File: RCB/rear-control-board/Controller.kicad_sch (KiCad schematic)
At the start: 26 parts, among them J6 Conn_01x05, U1 STM32F413CGUx, U2 LD1117S33TR_SOT223, U4 MCP2551-I-SN, Y1 Crystal

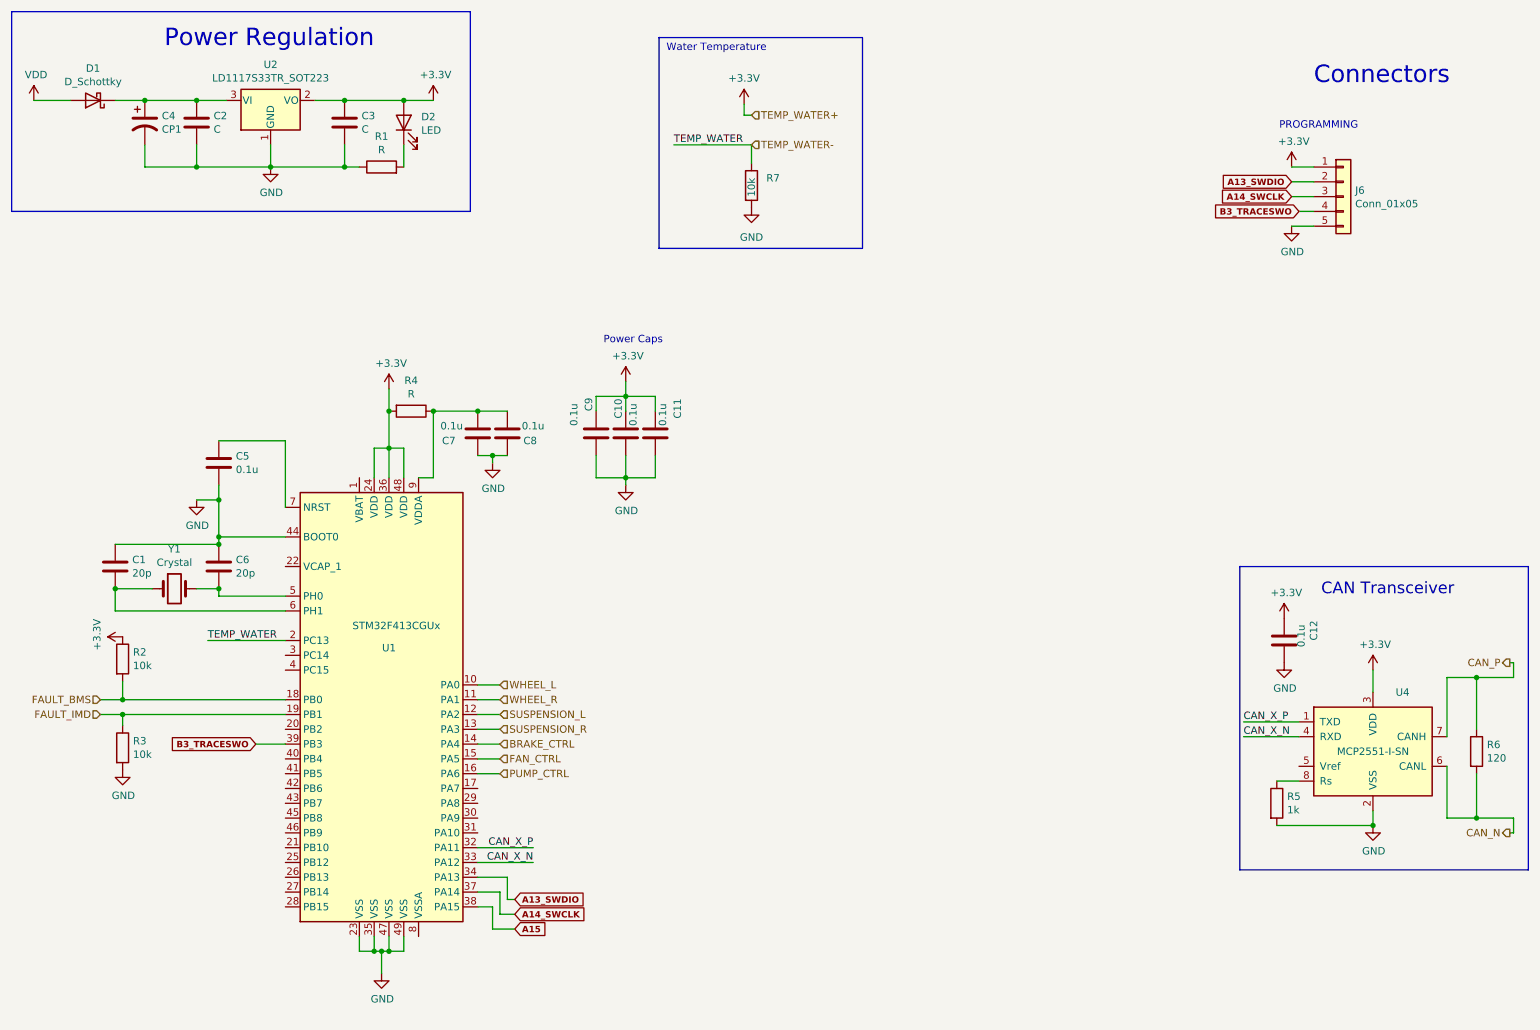
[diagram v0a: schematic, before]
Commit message: trace layout complete (need review)
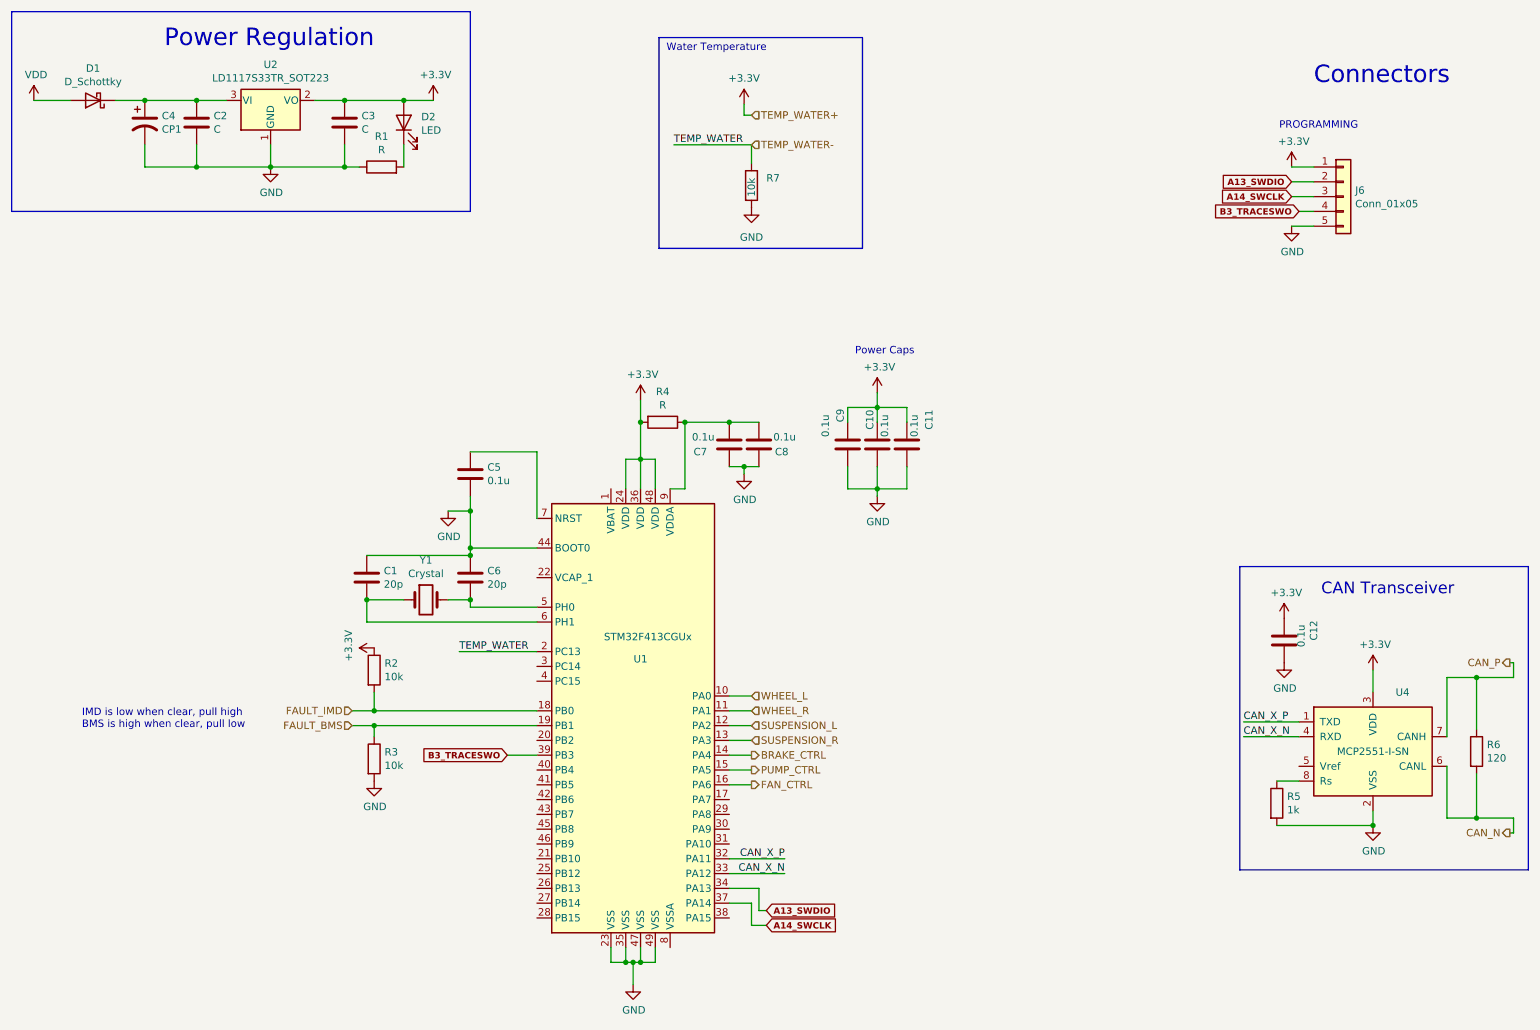
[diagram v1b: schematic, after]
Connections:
- net FAN_CTRL: now also U1.16 (PA6); no longer U1.15 (PA5)
- net FAULT_BMS: now also R3.1, U1.19 (PB1); no longer R2.2, U1.18 (PB0)
- net FAULT_IMD: now also R2.2, U1.18 (PB0); no longer R3.1, U1.19 (PB1)
- net PUMP_CTRL: now also U1.15 (PA5); no longer U1.16 (PA6)
- net A15: no longer names the net of U1.38 (PA15)
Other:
- note added: "IMD is low when clear, pull high BMS is high when clear, pull low"
- moved on the sheet: C1, C10, C11, C5, C6, C7, C8, C9, R2, R3, R4, U1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
